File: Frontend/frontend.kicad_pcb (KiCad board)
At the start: 4 copper layers, 100 x 100.2 mm, 342 parts, among them J1 SATA, J10 SWD, J11 APWR, J2 BNC, J3 SATA, J6 BNC, J9 PCIEx4 EDGE, K1 HE3600, K2 EE2-5NU, K3 HE3600, K4 HE3600, K5 EE2-5NU, K6 HE3600, Q1 ULN2003AD, U1 MCP9700T-E/TT, U10 ADA4817-1ACPZ, U11 MAX4567EEE, U12 MAX4567EEE, U13 MAX4567EEE, U14 AD8003ACPZ, U15 LMH6552SD, U16 MC33078DGK, U17 MAX5725AAUP, U18 STM32F030C8T, U19 MC33078DGK, U2 ADA4817-1ACPZ, U20 MC33078DGK, U23 LM317S, U24 MCP9700T-E/TT, U25 L78M05CDT, U26 TLV70233DSE, U27 MCP9700T-E/TT, U28 MC79M05CDT, U3 MAX4567EEE, U4 MAX4567EEE, U5 MAX4567EEE, U6 AD8003ACPZ, U7 LMH6552SD, U8 MC33078DGK, U9 MCP9700T-E/TT

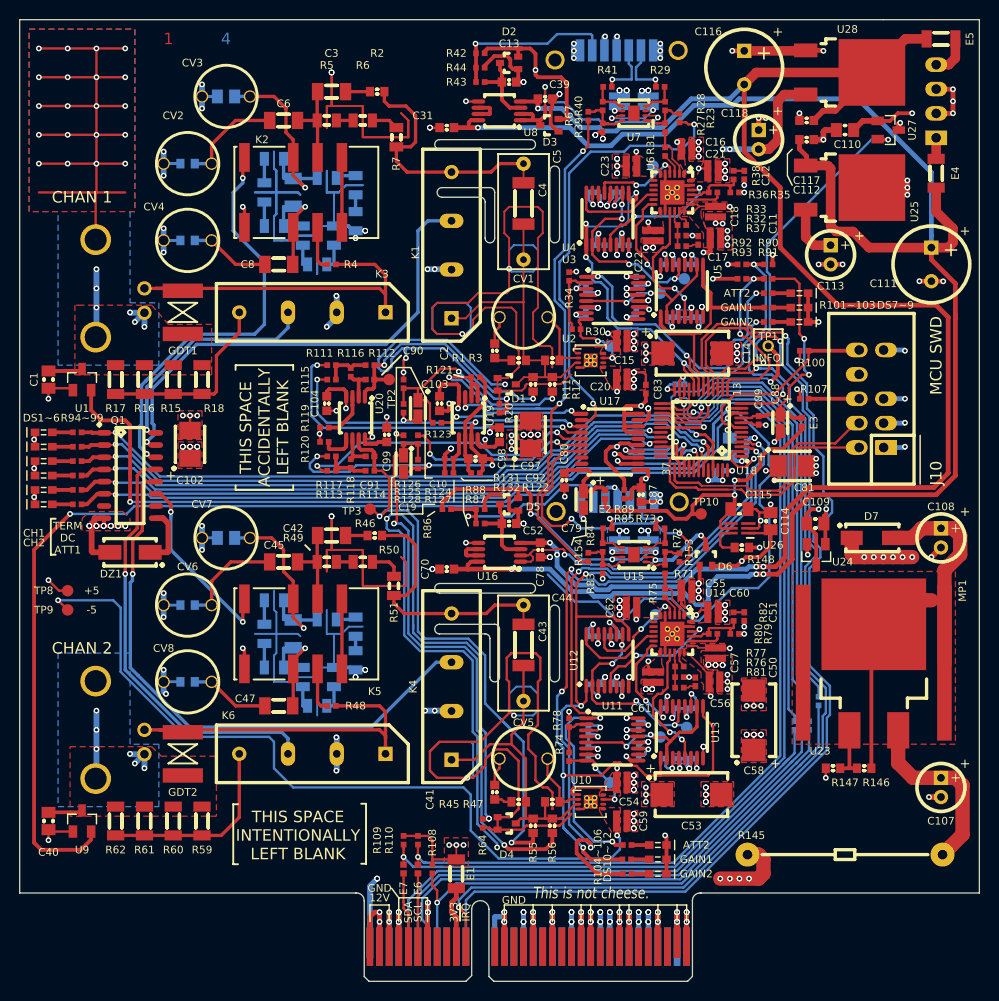
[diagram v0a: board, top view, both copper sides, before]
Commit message: More routing adjustments
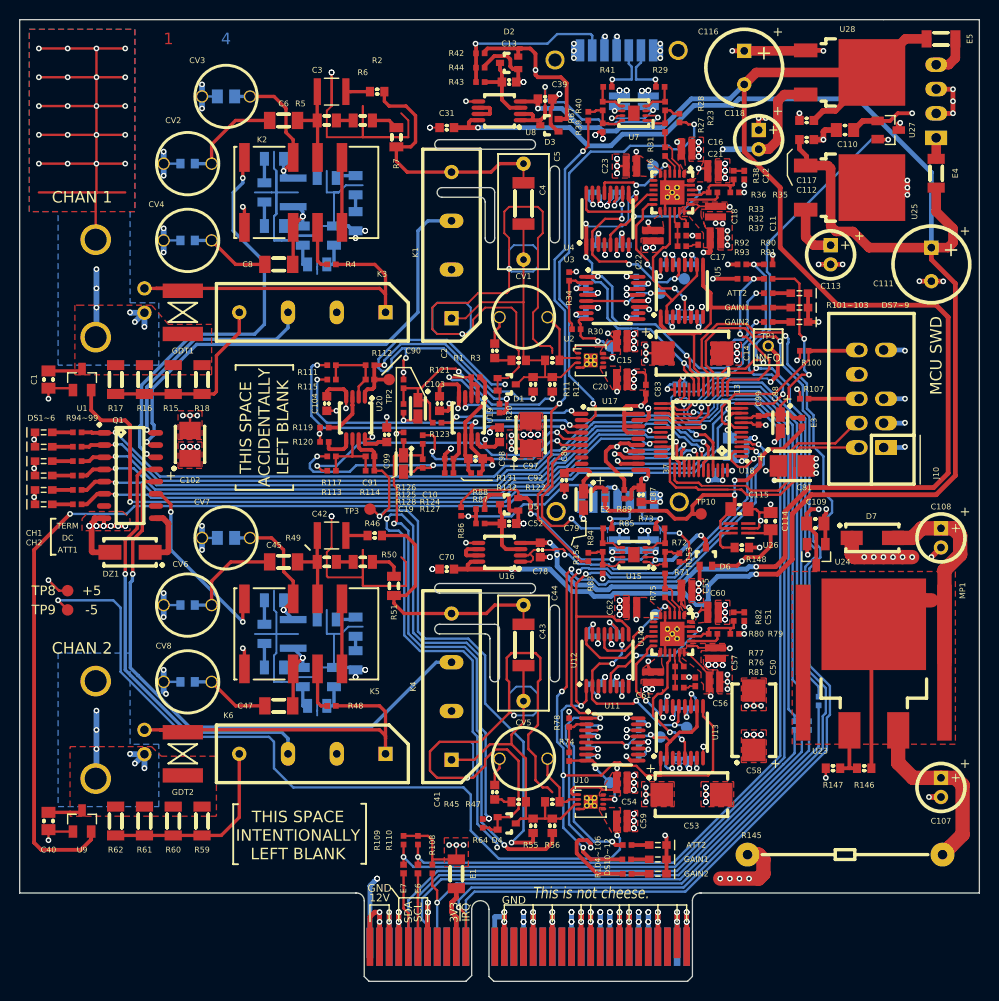
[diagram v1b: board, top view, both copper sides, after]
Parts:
- removed R116, R118: 5k6, IPC7351-Nominal:RESC1005X40
- C3, C42, C46, C7: footprint IPC7351-Nominal:CAPC3216X70 -> smd-non-ipc:CAPC2828X260
- R1, R2, R45, R46: value 75 -> 64R9
- R119, R120, R121, R122, R131, R132: value 5k6 -> 3k3
- R146: value 120 -> 165
- R147: value 430 -> 620
- R27, R39, R71, R83: value 150 -> 220
- R28, R31, R40, R43, R72, R75, R84, R87: value 443 -> 442
- R4, R48: value 33 -> 35R7
- moved R86 1.52 mm to (108.0, 69.2), turned to 270 degrees
- moved R127 0.50 mm to (104.0, 64.2)
- moved R124 0.50 mm to (104.0, 61.8)
- moved R128 0.30 mm to (102.0, 61.5)
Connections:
- R111 pad 1: Net-(R111-Pad1) -> Net-(C90-Pad2)
- R112 pad 2: Net-(R111-Pad1) -> Net-(C90-Pad2)
- R113 pad 1: Net-(R113-Pad1) -> Net-(C91-Pad2)
- R114 pad 2: Net-(R113-Pad1) -> Net-(C91-Pad2)
- R115 pad 1: Net-(R111-Pad1) -> Net-(C90-Pad2)
- R117 pad 1: Net-(R113-Pad1) -> Net-(C91-Pad2)
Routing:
- net GND: track 1325.5 -> 1128.9 mm
- net /Microcontroller/CH1_TEMP: track 155.3 -> 83.9 mm
- net VRELAY: track 253.6 -> 239.4 mm, vias 16 -> 8
- net /Channel1/GUARD: track 97.6 -> 86.5 mm
- net /Channel2/GUARD: track 97.0 -> 86.7 mm
- net Net-(C46-Pad1): track 21.6 -> 15.2 mm, vias 1 -> 2
- net Net-(C7-Pad1): track 22.1 -> 15.9 mm
- net +5: track 522.9 -> 517.3 mm
- net Net-(R113-Pad1): track 5.25 -> 0.00 mm
- net Net-(R111-Pad1): track 4.85 -> 0.00 mm
- net Net-(C90-Pad2): track 3.48 -> 8.20 mm
- net Net-(C91-Pad2): track 3.85 -> 7.90 mm
- net +8: track 246.6 -> 243.5 mm, vias 10 -> 9
- net Net-(C46-Pad2): track 12.9 -> 10.8 mm, vias 1 -> 2
- net /Channel2/VOCM: track 20.8 -> 19.0 mm
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
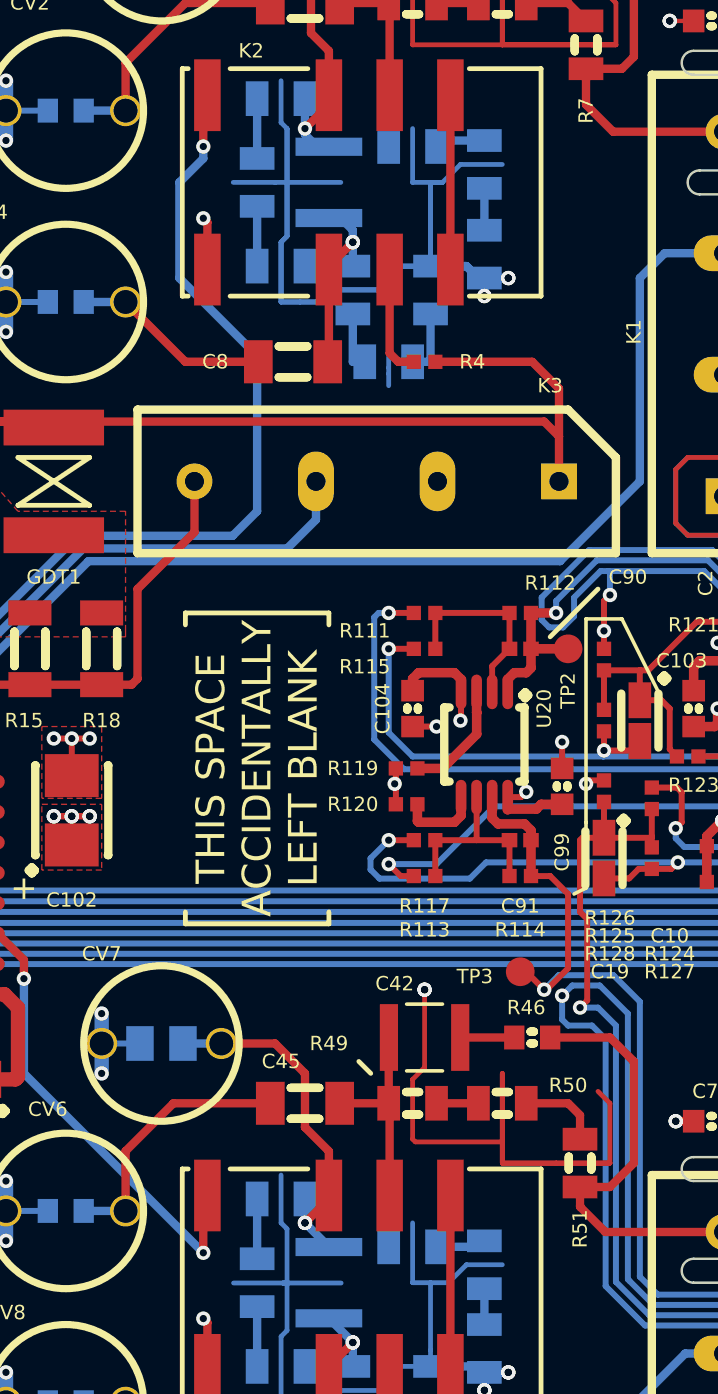
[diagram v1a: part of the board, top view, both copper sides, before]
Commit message: Update gerbers
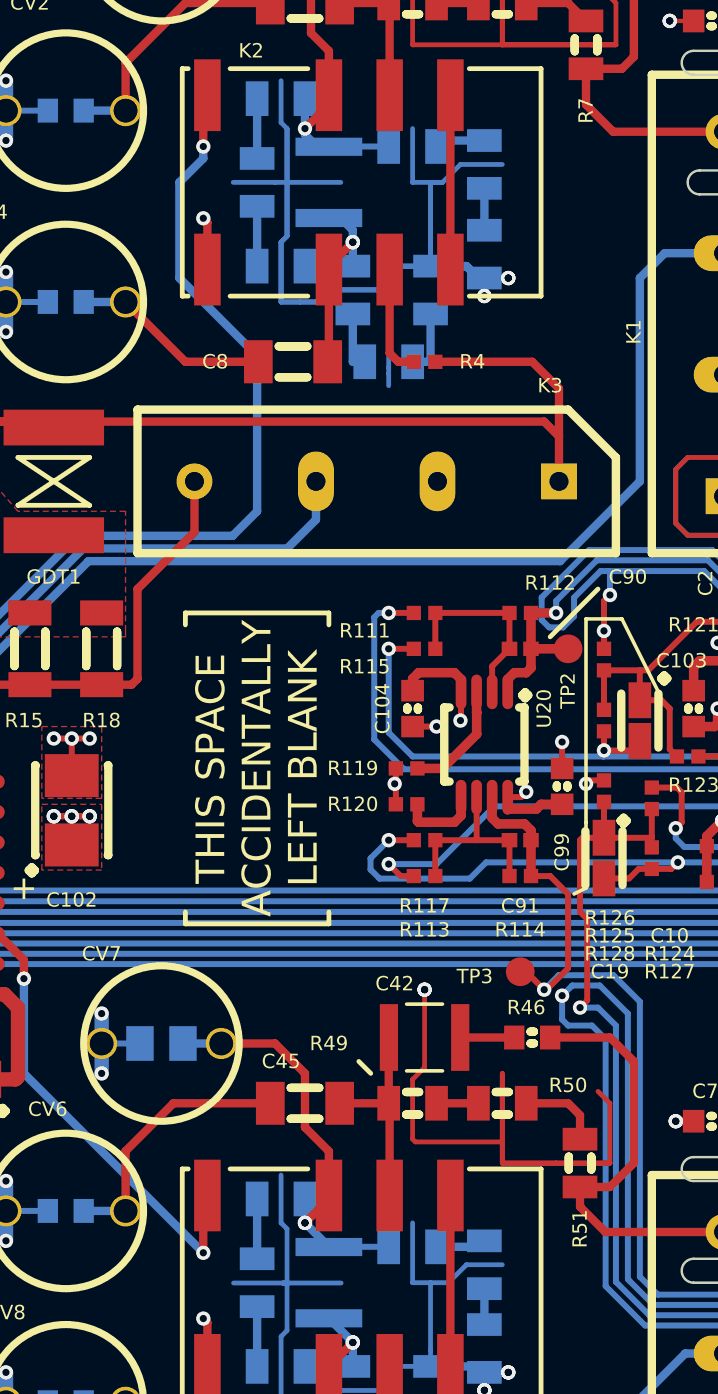
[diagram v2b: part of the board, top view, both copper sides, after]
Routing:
- net Net-(C7-Pad1): track 15.9 -> 18.4 mm
- net Net-(C46-Pad1): track 15.2 -> 17.7 mm
